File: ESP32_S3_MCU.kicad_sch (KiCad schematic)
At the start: 30 parts, among them SW1 SW_Push, SW2 SW_Push, U1 W25Q32JVSS, U2 ESP32-C3, X1 40MHz

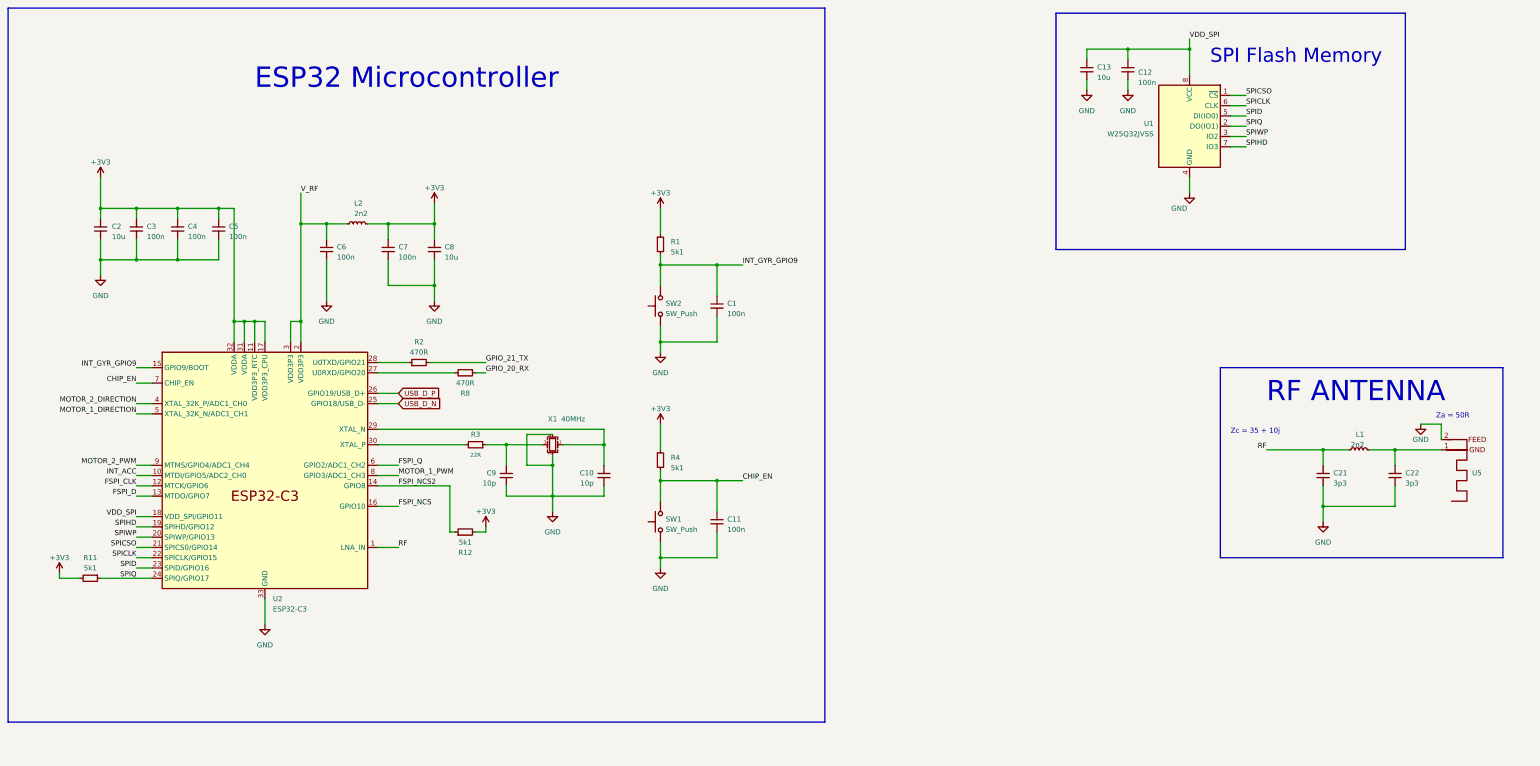
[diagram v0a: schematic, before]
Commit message: Update placement
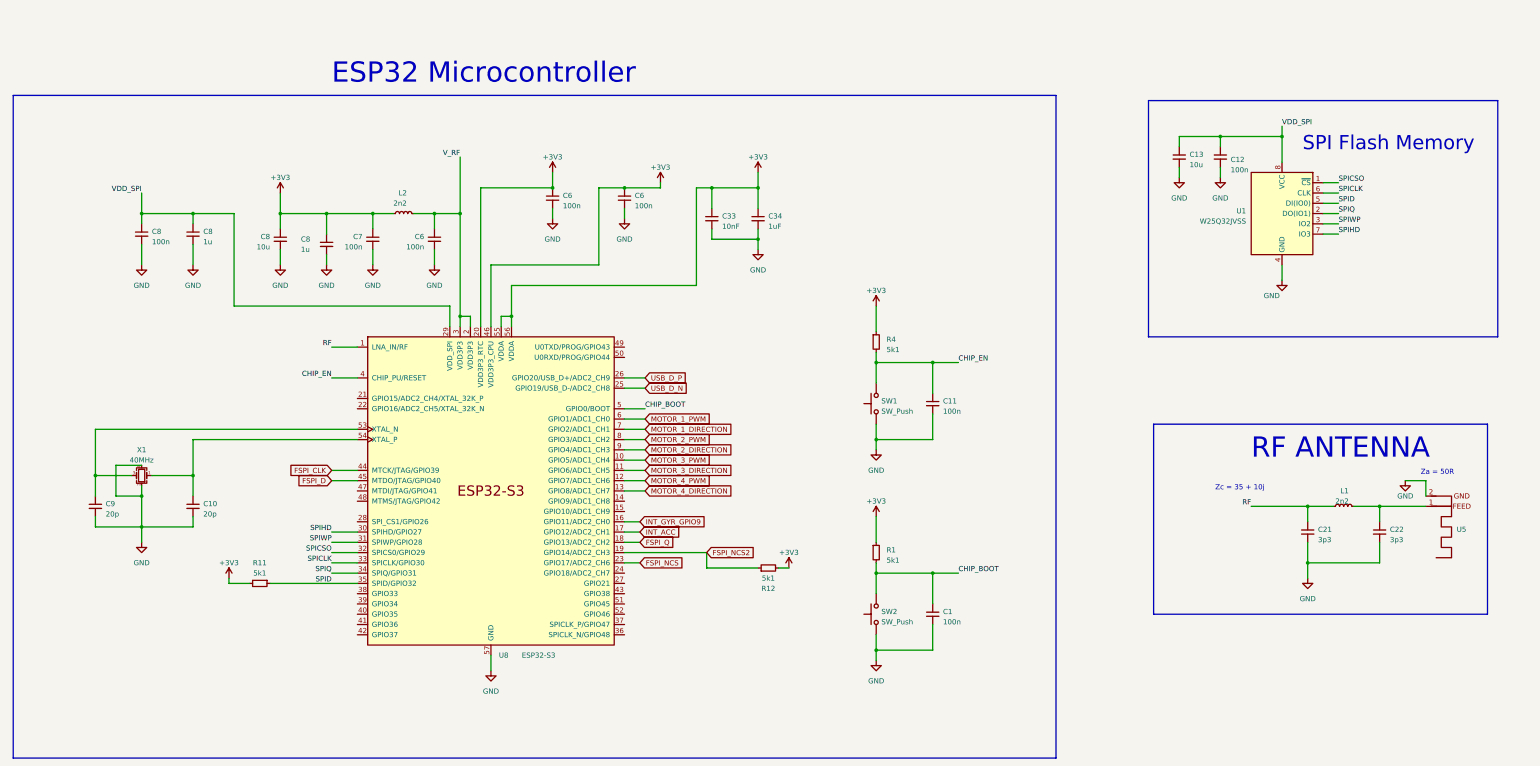
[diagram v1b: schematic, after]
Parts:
- removed C2: 10u, Capacitor_SMD:C_1210_3225Metric, symbol Device:C_Small
- removed C3, C4, C5, C6: 100n, Capacitor_SMD:C_0603_1608Metric, symbol Device:C_Small
- removed C8: 10u, Capacitor_SMD:C_0603_1608Metric, symbol Device:C_Small
- removed R2, R8: 470R, Resistor_SMD:R_0402_1005Metric, symbol Device:R_Small
- removed R3: 22R, Resistor_SMD:R_0402_1005Metric, symbol Device:R_Small
- removed U2: ESP32-C3, Package_DFN_QFN:QFN-32-1EP_5x5mm_P0.5mm_EP3.45x3.45mm, symbol PCM_Espressif:ESP32-C3
- added C33: 10nF, Capacitor_SMD:C_0402_1005Metric, symbol Device:C_Small
- added C34: 1uF, Capacitor_SMD:C_0402_1005Metric, symbol Device:C_Small
- added C6 (x3), C8: 100n, Capacitor_SMD:C_0402_1005Metric, symbol Device:C_Small
- added C8: 10u, Capacitor_SMD:C_0603_1608Metric, symbol Device:C_Small
- added C8 (x2): 1u, Capacitor_SMD:C_0402_1005Metric, symbol Device:C_Small
- added U8: ESP32-S3, Package_DFN_QFN:QFN-56-1EP_7x7mm_P0.4mm_EP5.6x5.6mm, symbol PCM_Espressif:ESP32-S3
- C1, C11, C12, C21, C22, C7: footprint Capacitor_SMD:C_0603_1608Metric -> Capacitor_SMD:C_0402_1005Metric
- C10, C9: value 10p -> 20p
- L1: footprint Inductor_SMD:L_0603_1608Metric -> Inductor_SMD:L_0402_1005Metric
- U5: footprint RF_Antenna:Texas_SWRA117D_2.4GHz_Right -> RF_Antenna:Texas_SWRA117D_2.4GHz_Left
- X1: footprint Crystal:Crystal_SMD_2520-4Pin_2.5x2.0mm -> KiCADv7:OSC_X322516MLB4SI; Field5 C255973 -> (none); LCSC (none) -> C13738
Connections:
- net +3V3: now also C33.1, C34.1, C6.1, C6.1, C8.1, C8.1, U8.20 (VDD3P3_RTC), U8.46 (VDD3P3_CPU), U8.55 (VDDA), U8.56 (VDDA)
- net CHIP_EN: now also U8.4 (CHIP_PU/RESET)
- net FSPI_CLK: now also U8.44 (MTCK/JTAG/GPIO39)
- net FSPI_D: now also U8.45 (MTDO/JTAG/GPIO40)
- net FSPI_NCS: now also U8.23 (GPIO17/ADC2_CH6)
- net FSPI_NCS2: now also U8.19 (GPIO14/ADC2_CH3)
- net FSPI_Q: now also U8.18 (GPIO13/ADC2_CH2)
- net GND: now also C33.2, C34.2, C6.2, C6.2, C6.2, C8.2, C8.2, C8.2, C8.2, U8.57 (GND)
- net INT_ACC: now also U8.17 (GPIO12/ADC2_CH1)
- net INT_GYR_GPIO9: now also U8.16 (GPIO11/ADC2_CH0); no longer C1.1, R1.2, SW2.2
- net MOTOR_1_DIRECTION: now also U8.7 (GPIO2/ADC1_CH1)
- net MOTOR_1_PWM: now also U8.6 (GPIO1/ADC1_CH0)
- net MOTOR_2_DIRECTION: now also U8.9 (GPIO4/ADC1_CH3)
- net MOTOR_2_PWM: now also U8.8 (GPIO3/ADC1_CH2)
- net RF: now also U8.1 (LNA_IN/RF)
- net SPICLK: now also U8.33 (SPICLK/GPIO30)
- net SPICSO: now also U8.32 (SPICS0/GPIO29)
- net SPID: now also R11.1, U8.35 (SPID/GPIO32)
- net SPIHD: now also U8.30 (SPIHD/GPIO27)
- net SPIQ: now also U8.34 (SPIQ/GPIO31); no longer R11.1
- net SPIWP: now also U8.31 (SPIWP/GPIO28)
- net USB_D_N: now also U8.25 (GPIO19/USB_D-/ADC2_CH8)
- net USB_D_P: now also U8.26 (GPIO20/USB_D+/ADC2_CH9)
- net VDD_SPI: now also C8.1, C8.1, U8.29 (VDD_SPI)
- net V_RF: now also C6.1, U8.2 (VDD3P3), U8.3 (VDD3P3)
- net at C9.1, X1.3: now also U8.53 (XTAL_N)
- net at C10.1, X1.1: now also U8.54 (XTAL_P)
- new net CHIP_BOOT: C1.1, R1.2, SW2.2, U8.5 (GPIO0/BOOT)
- new net MOTOR_3_DIRECTION: U8.11 (GPIO6/ADC1_CH5)
- new net MOTOR_3_PWM: U8.10 (GPIO5/ADC1_CH4)
- new net MOTOR_4_DIRECTION: U8.13 (GPIO8/ADC1_CH7)
- new net MOTOR_4_PWM: U8.12 (GPIO7/ADC1_CH6)
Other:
- moved on the sheet: C12, C13, C21, C22, L1, U1, U5
